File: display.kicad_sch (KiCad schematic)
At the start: 17 parts, among them J5 LCD, Q3 BSS138, Q4 BSS138

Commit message: Fixed and added LCSC reference numbers for all components
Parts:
- R33, R38: MPN (none) -> 0402WGF1000TCE; PN 0402WGF1000TCE -> (none)
- R34, R36: MPN (none) -> 0402WGF1002TCE; PN 0402WGF1002TCE -> (none)
- R35, R39: MPN (none) -> 0402WGF4702TCE; PN 0402WGF4702TCE -> (none)
- R37: MPN (none) -> 0402WGF100JTCE; PN 0402WGF100JTCE -> (none)
- R40, R41: MPN (none) -> 0402WGF2200TCE; PN 0402WGF2200TCE -> (none)
- R42: MPN (none) -> 0402WGF1500TCE; PN 0402WGF1500TCE -> (none)
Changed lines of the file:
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@@
 			)
 		)
-		(property "PN" "0402WGF2200TCE"
+		(property "PN" ""
 			(at 219.71 68.58 90)
 			(effects
@@
 		)
 		(property "LCSC Part" ""
+			(at 219.71 68.58 90)
+			(effects
+				(font
+					(size 1.27 1.27)
+				)
+				(hide yes)
+			)
+		)
+		(property "MPN" "0402WGF2200TCE"
 			(at 219.71 68.58 90)
 			(effects
@@
 			)
 		)
-		(property "PN" "0402WGF1002TCE"
+		(property "PN" ""
 			(at 101.6 82.55 0)
 			(effects
@@
 		)
 		(property "LCSC Part" ""
+			(at 101.6 82.55 0)
+			(effects
+				(font
+					(size 1.27 1.27)
+				)
+				(hide yes)
+			)
+		)
+		(property "MPN" "0402WGF1002TCE"
 			(at 101.6 82.55 0)
 			(effects
@@
 			)
 		)
-		(property "PN" "0402WGF4702TCE"
+		(property "PN" ""
 			(at 101.6 134.62 0)
 			(effects
@@
 		)
 		(property "LCSC Part" ""
+			(at 101.6 134.62 0)
+			(effects
+				(font
+					(size 1.27 1.27)
+				)
+				(hide yes)
+			)
+		)
+		(property "MPN" "0402WGF4702TCE"
 			(at 101.6 134.62 0)
 			(effects
@@
 			)
 		)
-		(property "PN" "0402WGF1000TCE"
+		(property "PN" ""
 			(at 185.42 99.06 90)
 			(effects
@@
 		)
 		(property "LCSC Part" ""
+			(at 185.42 99.06 90)
+			(effects
+				(font
+					(size 1.27 1.27)
+				)
+				(hide yes)
+			)
+		)
+		(property "MPN" "0402WGF1000TCE"
 			(at 185.42 99.06 90)
 			(effects
@@
 			)
 		)
-		(property "PN" "0402WGF100JTCE"
+		(property "PN" ""
 			(at 111.76 116.84 0)
 			(effects
@@
 		)
 		(property "LCSC Part" ""
+			(at 111.76 116.84 0)
+			(effects
+				(font
+					(size 1.27 1.27)
+				)
+				(hide yes)
+			)
+		)
+		(property "MPN" "0402WGF100JTCE"
 			(at 111.76 116.84 0)
 			(effects
@@
 			)
 		)
-		(property "PN" "0402WGF4702TCE"
+		(property "PN" ""
 			(at 191.77 105.41 0)
 			(effects
@@
 		)
 		(property "LCSC Part" ""
+			(at 191.77 105.41 0)
+			(effects
+				(font
+					(size 1.27 1.27)
+				)
+				(hide yes)
+			)
+		)
+		(property "MPN" "0402WGF4702TCE"
 			(at 191.77 105.41 0)
 			(effects
@@
 			)
 		)
-		(property "PN" "0402WGF1500TCE"
+		(property "PN" ""
 			(at 219.71 90.17 90)
 			(effects
@@
 		)
 		(property "LCSC Part" ""
+			(at 219.71 90.17 90)
+			(effects
+				(font
+					(size 1.27 1.27)
+				)
+				(hide yes)
+			)
+		)
+		(property "MPN" "0402WGF1500TCE"
 			(at 219.71 90.17 90)
 			(effects
@@
 			)
 		)
-		(property "PN" "0402WGF2200TCE"
+		(property "PN" ""
 			(at 219.71 80.01 90)
 			(effects
@@
 		)
 		(property "LCSC Part" ""
+			(at 219.71 80.01 90)
+			(effects
+				(font
+					(size 1.27 1.27)
+				)
+				(hide yes)
+			)
+		)
+		(property "MPN" "0402WGF2200TCE"
 			(at 219.71 80.01 90)
 			(effects
@@
 			)
 		)
-		(property "PN" "0402WGF1002TCE"
+		(property "PN" ""
 			(at 102.87 64.77 90)
 			(effects
@@
 		)
 		(property "LCSC Part" ""
+			(at 102.87 64.77 90)
+			(effects
+				(font
+					(size 1.27 1.27)
+				)
+				(hide yes)
+			)
+		)
+		(property "MPN" "0402WGF1002TCE"
 			(at 102.87 64.77 90)
 			(effects
@@
 			)
 		)
-		(property "PN" "0402WGF1000TCE"
+		(property "PN" ""
 			(at 95.25 128.27 90)
 			(effects
@@
 			(at 95.25 128.27 90)
 			(effects
+				(font
+					(size 1.27 1.27)
+				)
+				(hide yes)
+			)
+		)
+		(property "MPN" "0402WGF1000TCE"
+			(at 95.25 128.27 90)
+			(effects

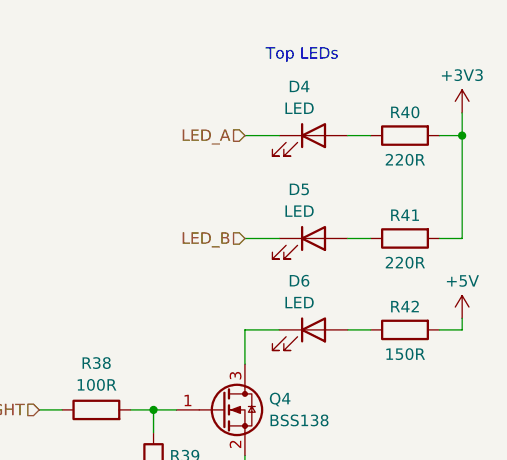
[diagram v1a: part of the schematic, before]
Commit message: Changed LED resistors from 220R to 100R
Fixes #37
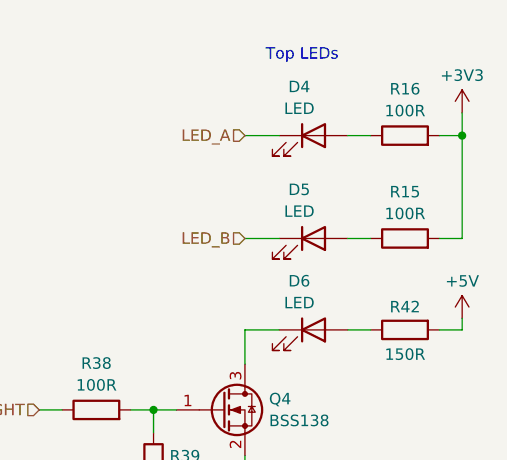
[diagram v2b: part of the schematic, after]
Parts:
- removed R40, R41: 220R, Resistor_SMD:R_0402_1005Metric, symbol Device:R
- added R15, R16: 100R, Resistor_SMD:R_0402_1005Metric, symbol Device:R
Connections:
- net +3V3: now also R15.2, R16.2
- net at D4.2 (A): now also R16.1
- net at D5.2 (A): now also R15.1
